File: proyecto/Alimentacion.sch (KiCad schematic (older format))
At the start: 9 parts

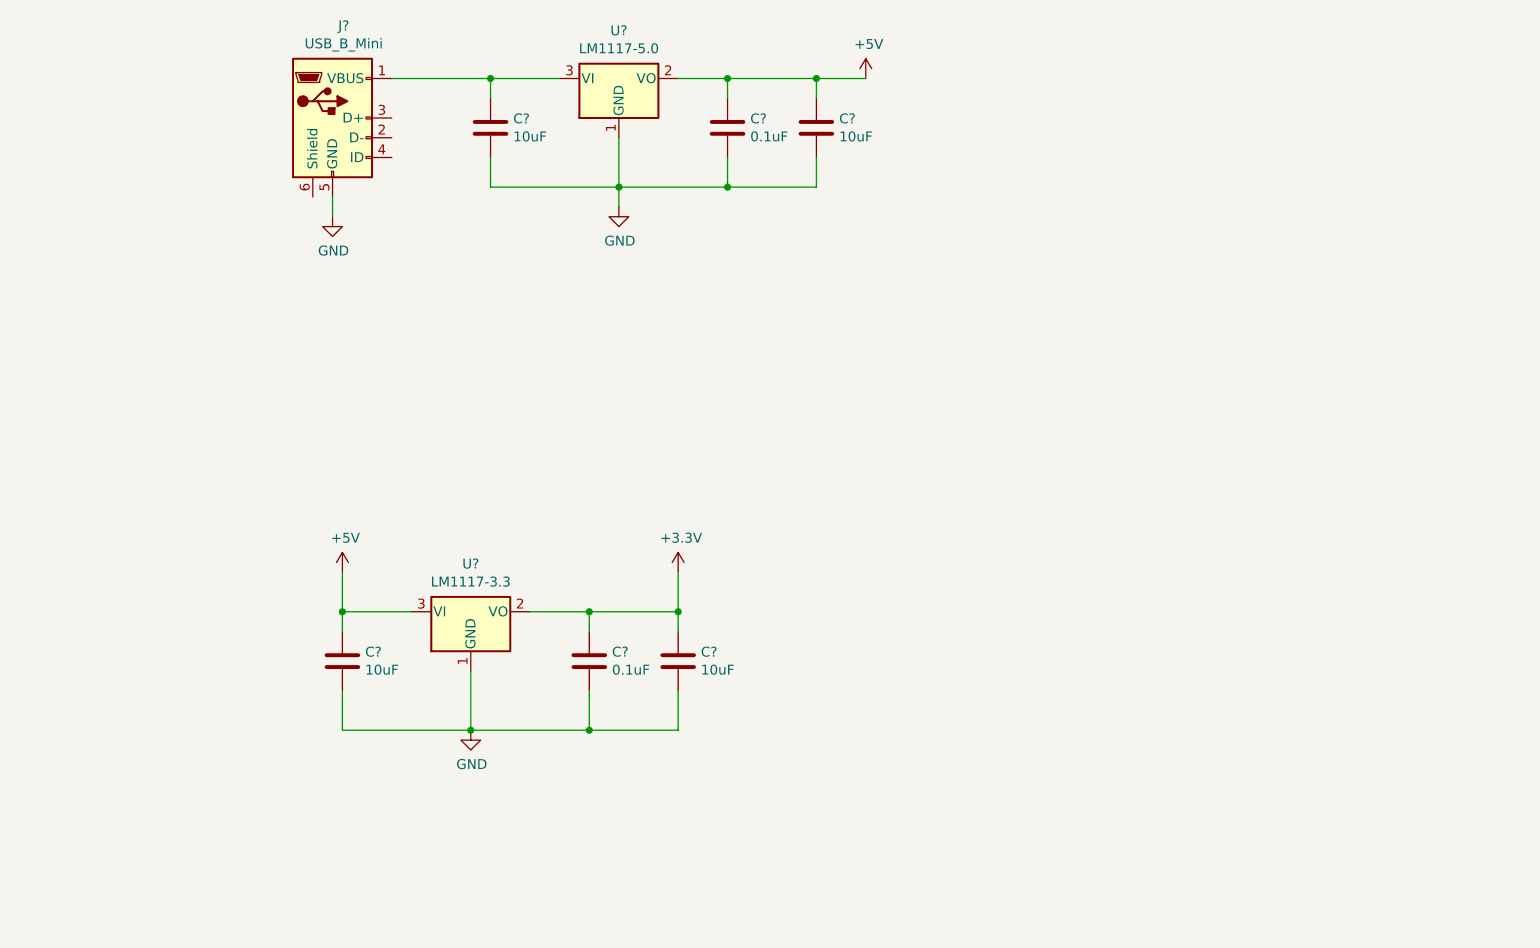
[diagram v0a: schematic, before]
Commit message: Add files via upload
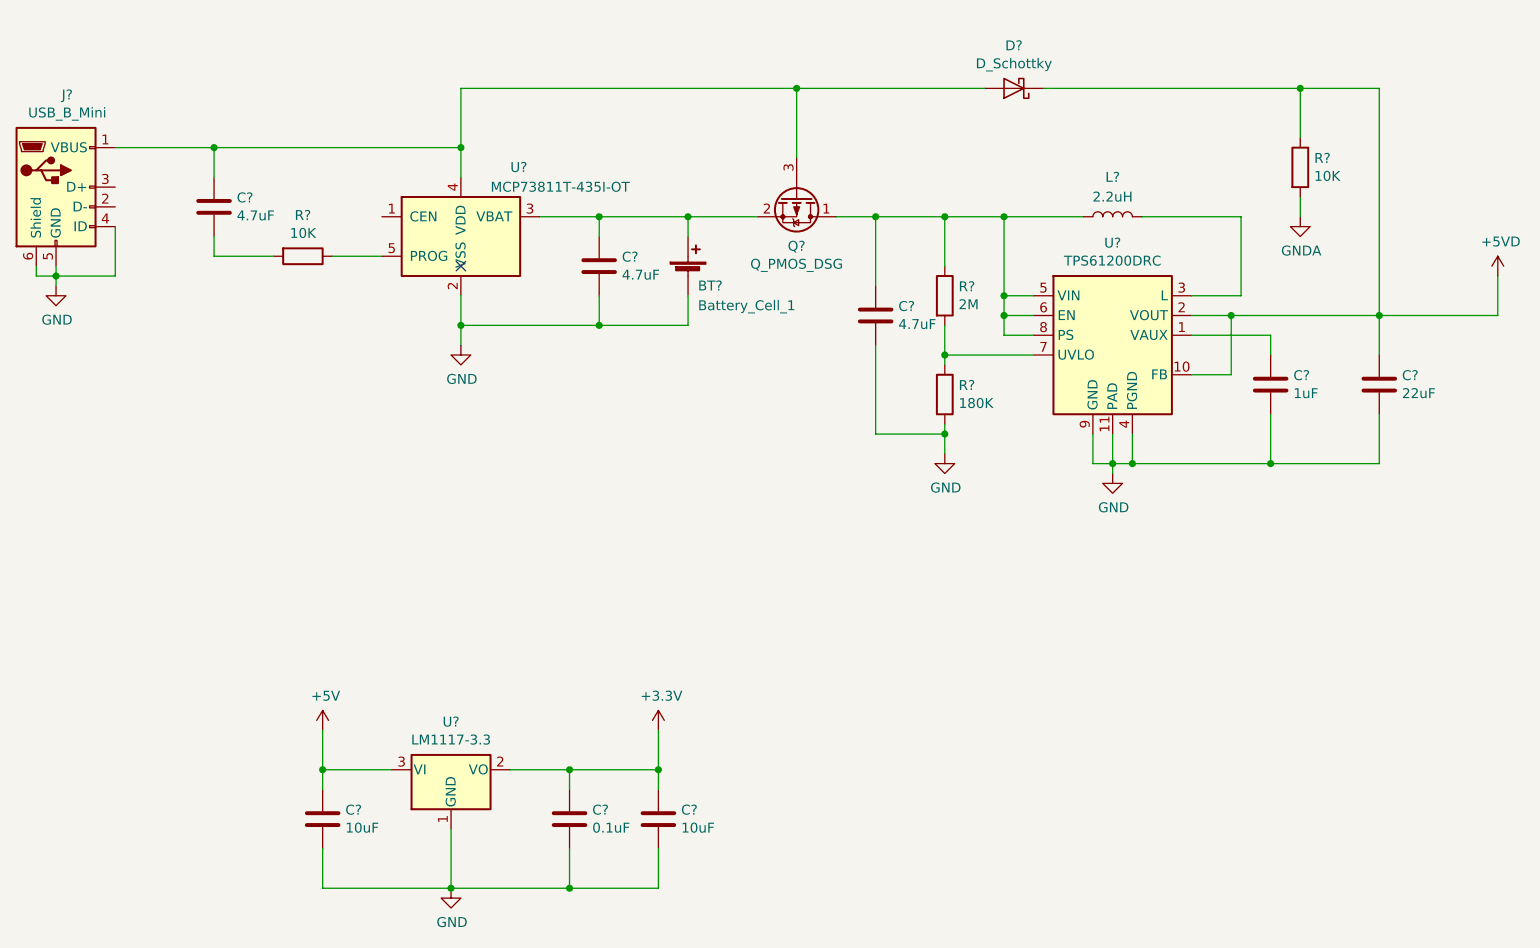
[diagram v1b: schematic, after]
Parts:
- removed C?: 0.1uF, symbol Device:C
- removed C? (x2): 10uF, symbol Device:C
- removed J?: USB_B_Mini, symbol Connector:USB_B_Mini
- removed U?: LM1117-5.0, symbol Regulator_Linear:LM1117-5.0
- added BT?: Battery_Cell_1, symbol Device:Battery_Cell
- added C? (x3): 4.7uF, symbol Device:C
- added C?: 1uF, symbol Device:C
- added C?: 22uF, symbol Device:C
- added D?: D_Schottky, symbol Device:D_Schottky
- added J?: USB_B_Mini, symbol Connector:USB_B_Mini
- added L?: 2.2uH, symbol Device:L
- added Q?: Q_PMOS_DSG, symbol Device:Q_PMOS_DSG
- added R? (x2): 10K, symbol Device:R
- added R?: 2M, symbol Device:R
- added R?: 180K, symbol Device:R
- added U?: MCP73811T-435I-OT, Package_TO_SOT_SMD:SOT-23-5, symbol Battery_Management:MCP73811T-435I-OT
- added U?: TPS61200DRC, Package_SON:Texas_S-PVSON-N10_ThermalVias, symbol Regulator_Switching:TPS61200DRC
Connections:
- net GND: now also BT?.2 (-), C?.2, C?.2, C?.2, C?.2, J?.4 (ID), J?.5 (GND), J?.6 (Shield), R?.2, U?.11 (PAD), U?.2 (VSS), U?.4 (PGND), U?.9 (GND)
- new net: C?.1, D?.2 (A), J?.1 (VBUS), Q?.3 (G), U?.4 (VDD)
- new net: C?.2, R?.2
- new net: R?.1, U?.5 (PROG)
- new net: BT?.1 (+), C?.1, Q?.2 (S), U?.3 (VBAT)
- new net: C?.1, L?.1, Q?.1 (D), R?.1, U?.5 (VIN), U?.6 (EN), U?.8 (PS)
- new net: C?.1, U?.1 (VAUX)
- new net: L?.2, U?.3 (L)
- new net: R?.1, R?.2, U?.7 (UVLO)
- new net +5VD: C?.1, D?.1 (K), R?.1, U?.10 (FB), U?.2 (VOUT)
- new net GNDA: R?.2
- no-connect marks 0 -> 1
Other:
- moved on the sheet: C?, U?
